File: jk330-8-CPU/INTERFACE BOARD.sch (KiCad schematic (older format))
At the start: 33 parts, among them U2001 74C922, U2002 PCF8574T, U2003 74LS20

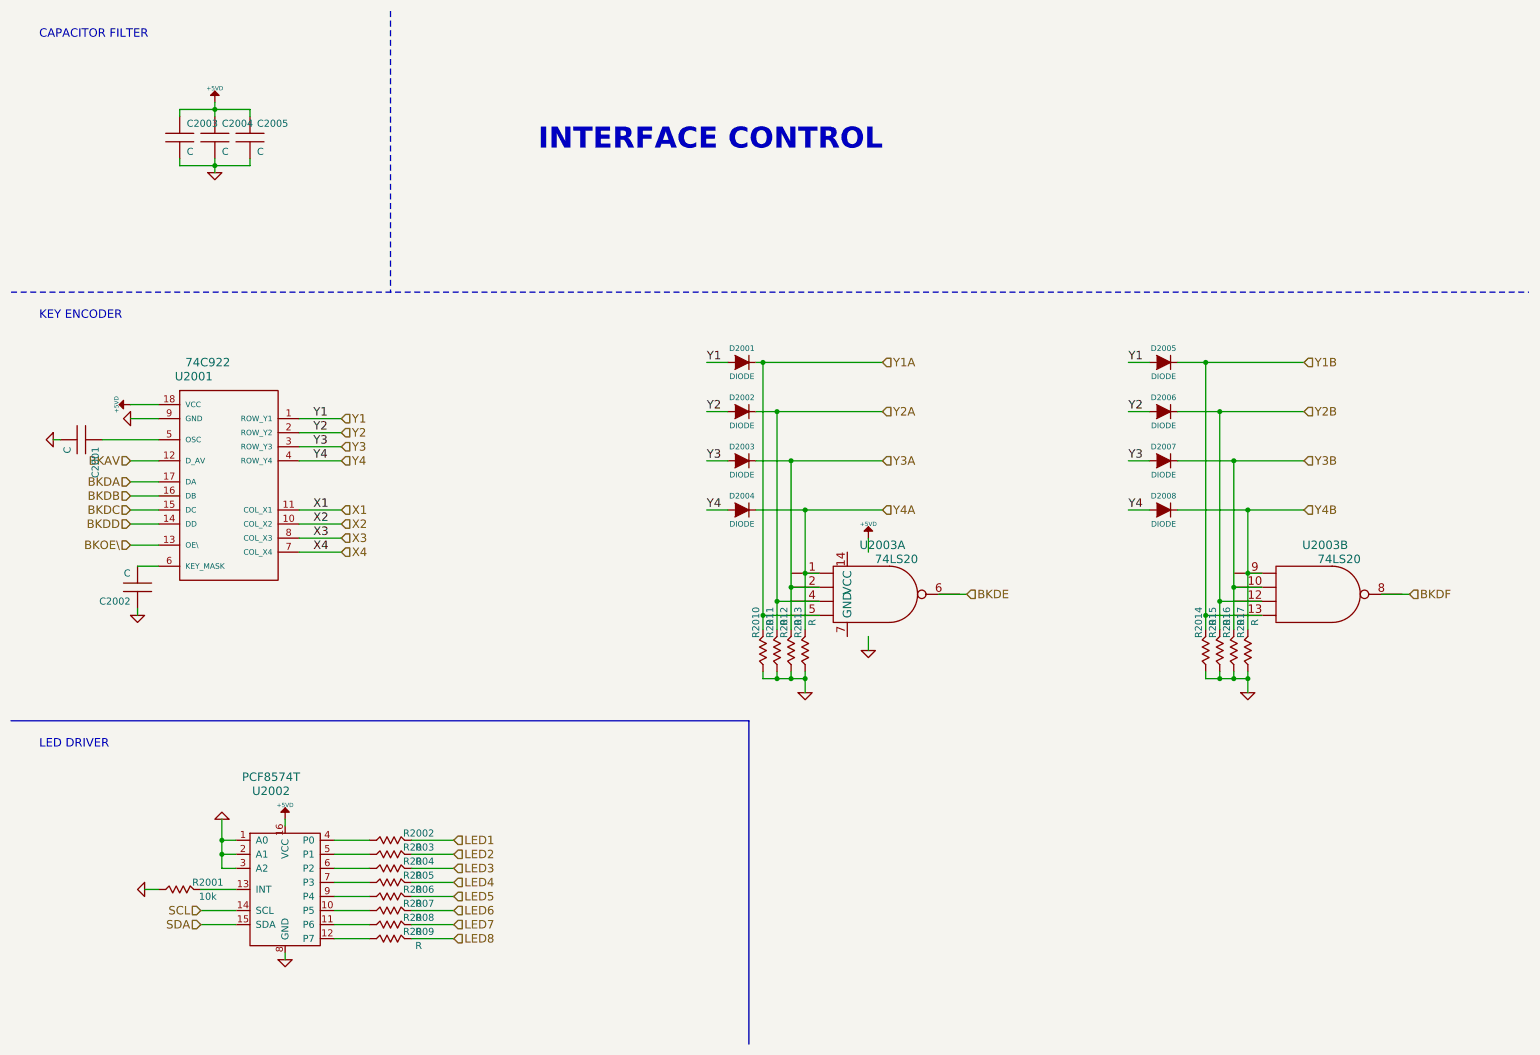
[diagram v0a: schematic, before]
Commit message: CPU SCHEMA 100%
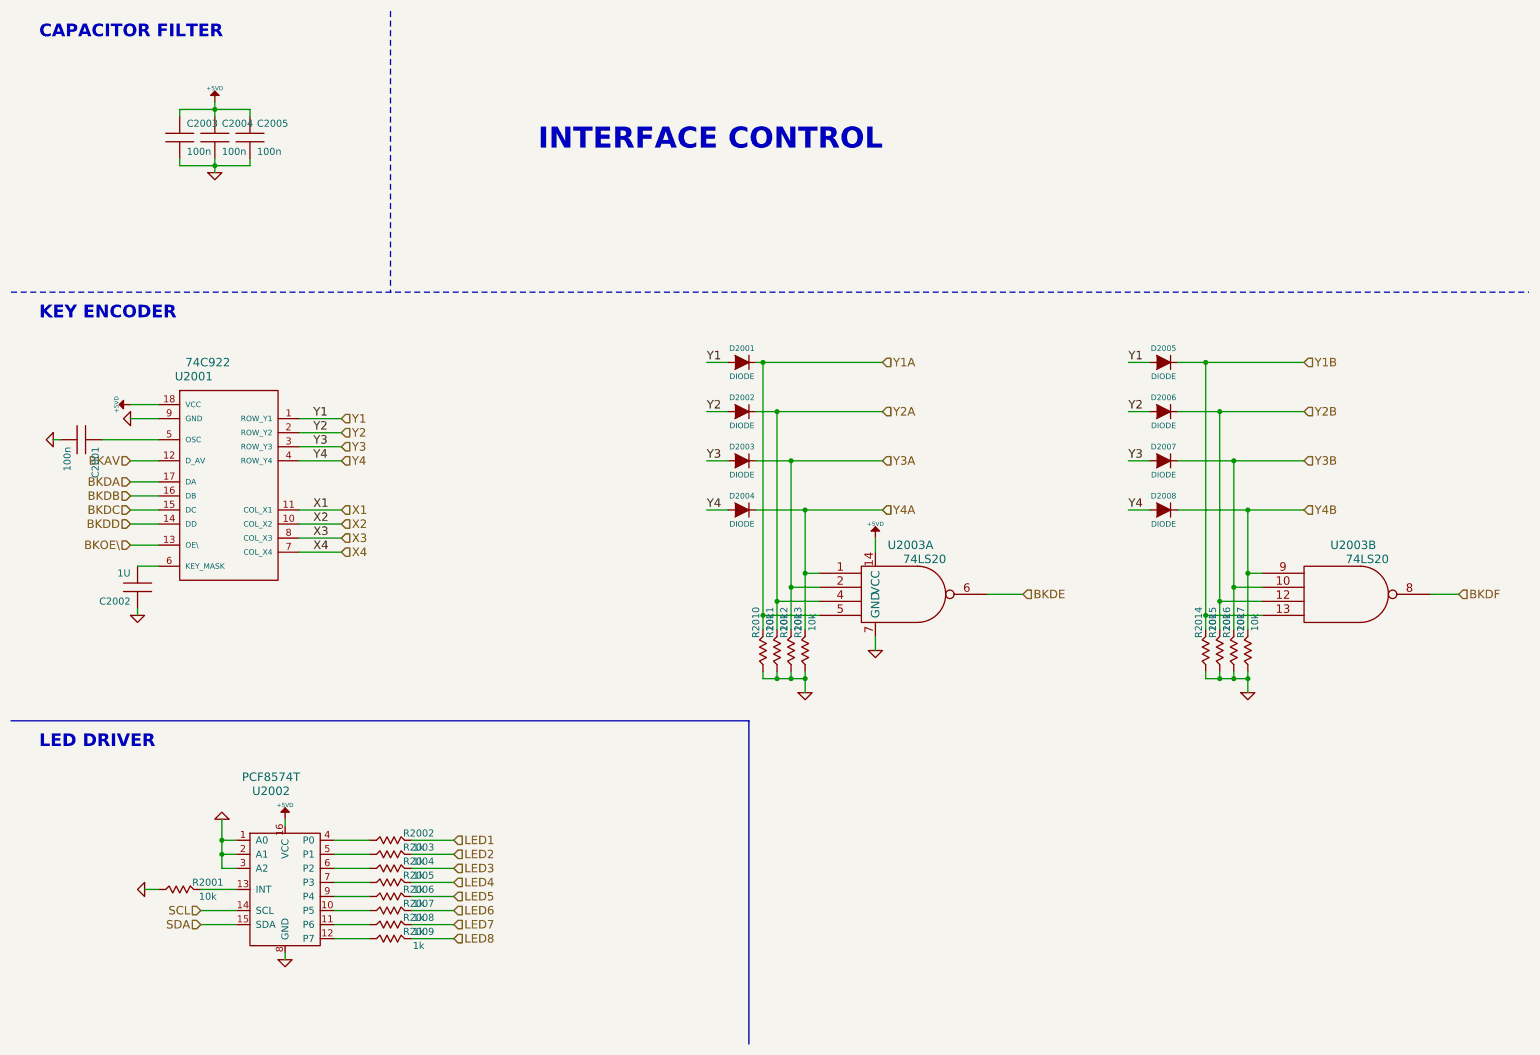
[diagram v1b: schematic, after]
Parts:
- C2001, C2003, C2004, C2005: value C -> 100n
- C2002: value C -> 1U
- R2002, R2003, R2004, R2005, R2006, R2007, R2008, R2009: value R -> 1k
- R2010, R2011, R2012, R2013, R2014, R2015, R2016, R2017: value R -> 10k
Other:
- moved on the sheet: U2003A, U2003B
